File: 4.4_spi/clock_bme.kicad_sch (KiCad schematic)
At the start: 9 parts, among them U1 ESP32-S3-DevKitC, U2 DS18B20, U3 DS1307+, U4 SSD1306, U5 BME280, Y1 Crystal

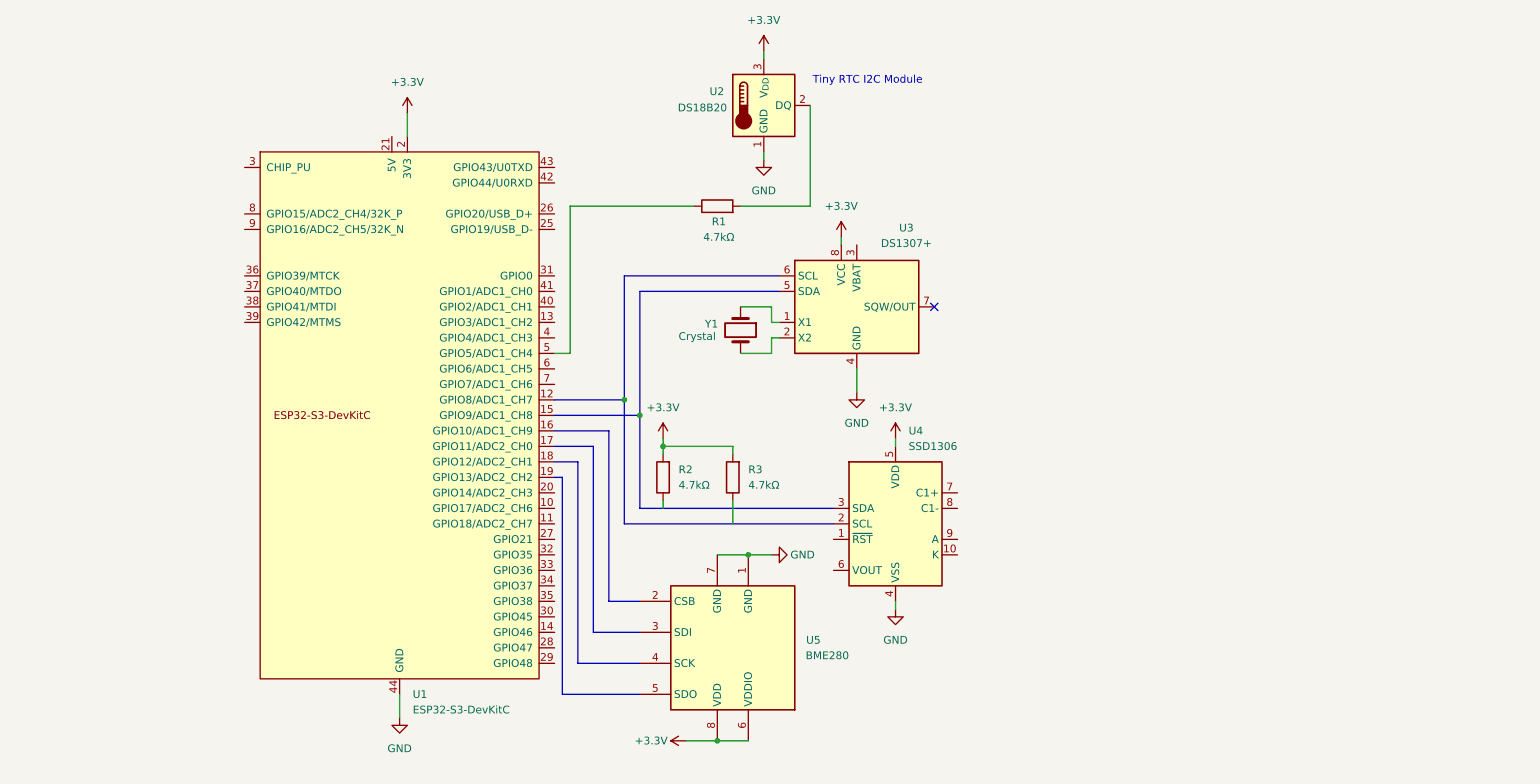
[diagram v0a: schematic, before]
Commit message: added HW4.4 - previous
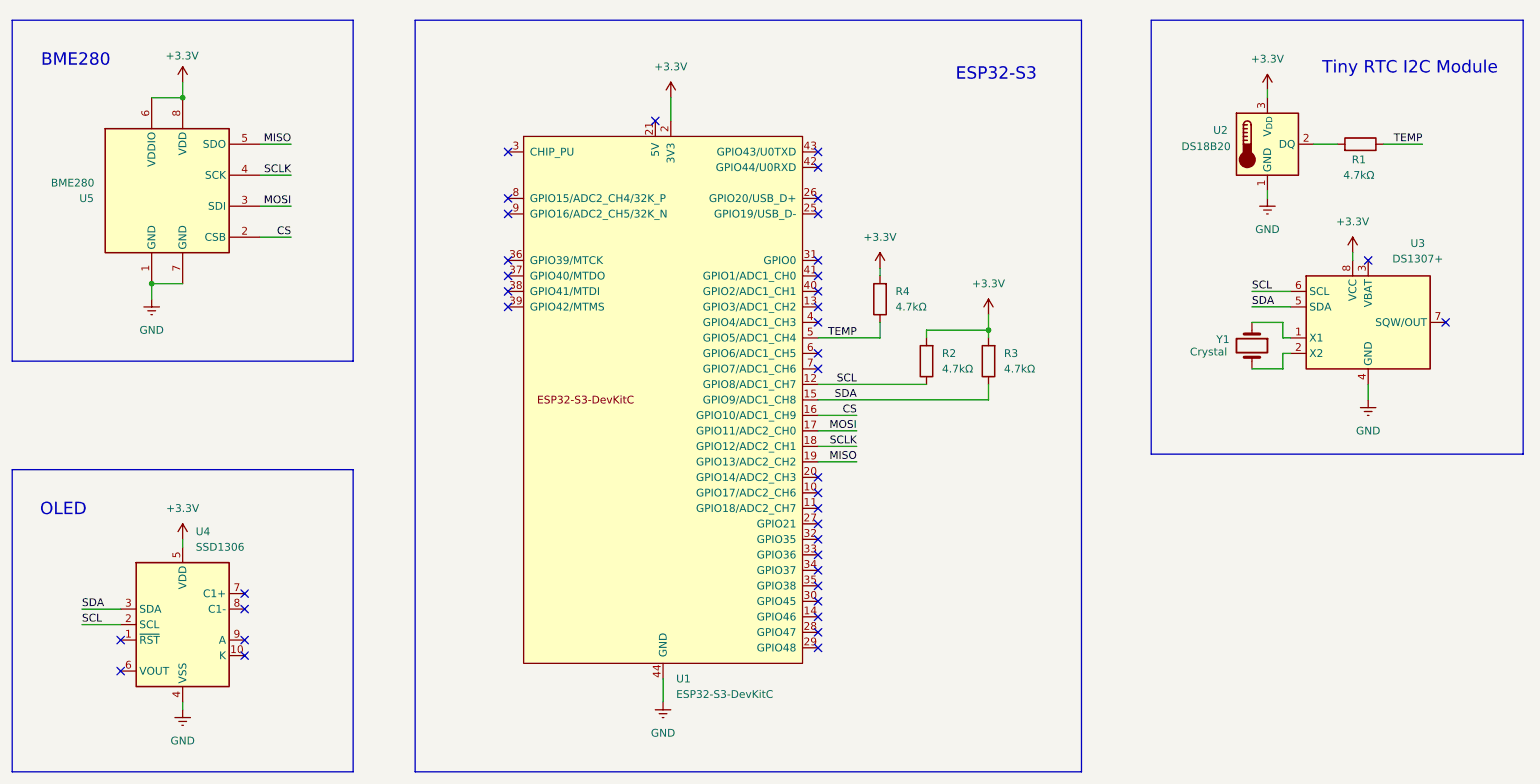
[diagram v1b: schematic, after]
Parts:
- added R4: 4.7kΩ, symbol Device:R
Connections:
- net +3.3V: now also R4.2
- net SCL: now reaches R2.1
- net SCL: now also U1.12 (GPIO8/ADC1_CH7), U3.6 (SCL), U4.2 (SCL)
- net CS: now reaches U5.2 (CSB)
- net CS: now also U1.16 (GPIO10/ADC1_CH9)
- net MOSI: now reaches U5.3 (SDI)
- net MOSI: now also U1.17 (GPIO11/ADC2_CH0)
- net SCLK: now reaches U5.4 (SCK)
- net SCLK: now also U1.18 (GPIO12/ADC2_CH1)
- net MISO: now reaches U5.5 (SDO)
- net MISO: now also U1.19 (GPIO13/ADC2_CH2)
- net TEMP: now reaches R1.1, U1.5 (GPIO5/ADC1_CH4)
- net TEMP: now also R4.1
- net SDA: now reaches U3.5 (SDA)
- net SDA: now also R3.1, U1.15 (GPIO9/ADC1_CH8), U4.3 (SDA)
- no-connect marks 1 -> 39
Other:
- note added: "BME280"
- note added: "ESP32-S3"
- note added: "OLED"
- moved on the sheet: R1, R2, R3, U1, U2, U3, U4, U5, Y1
